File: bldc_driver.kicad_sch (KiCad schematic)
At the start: 9 parts, among them IC1 TMC6200-TA, Q1 TPH1R306PL, Q2 TPH1R306PL, Q3 TPH1R306PL, Q4 TPH1R306PL

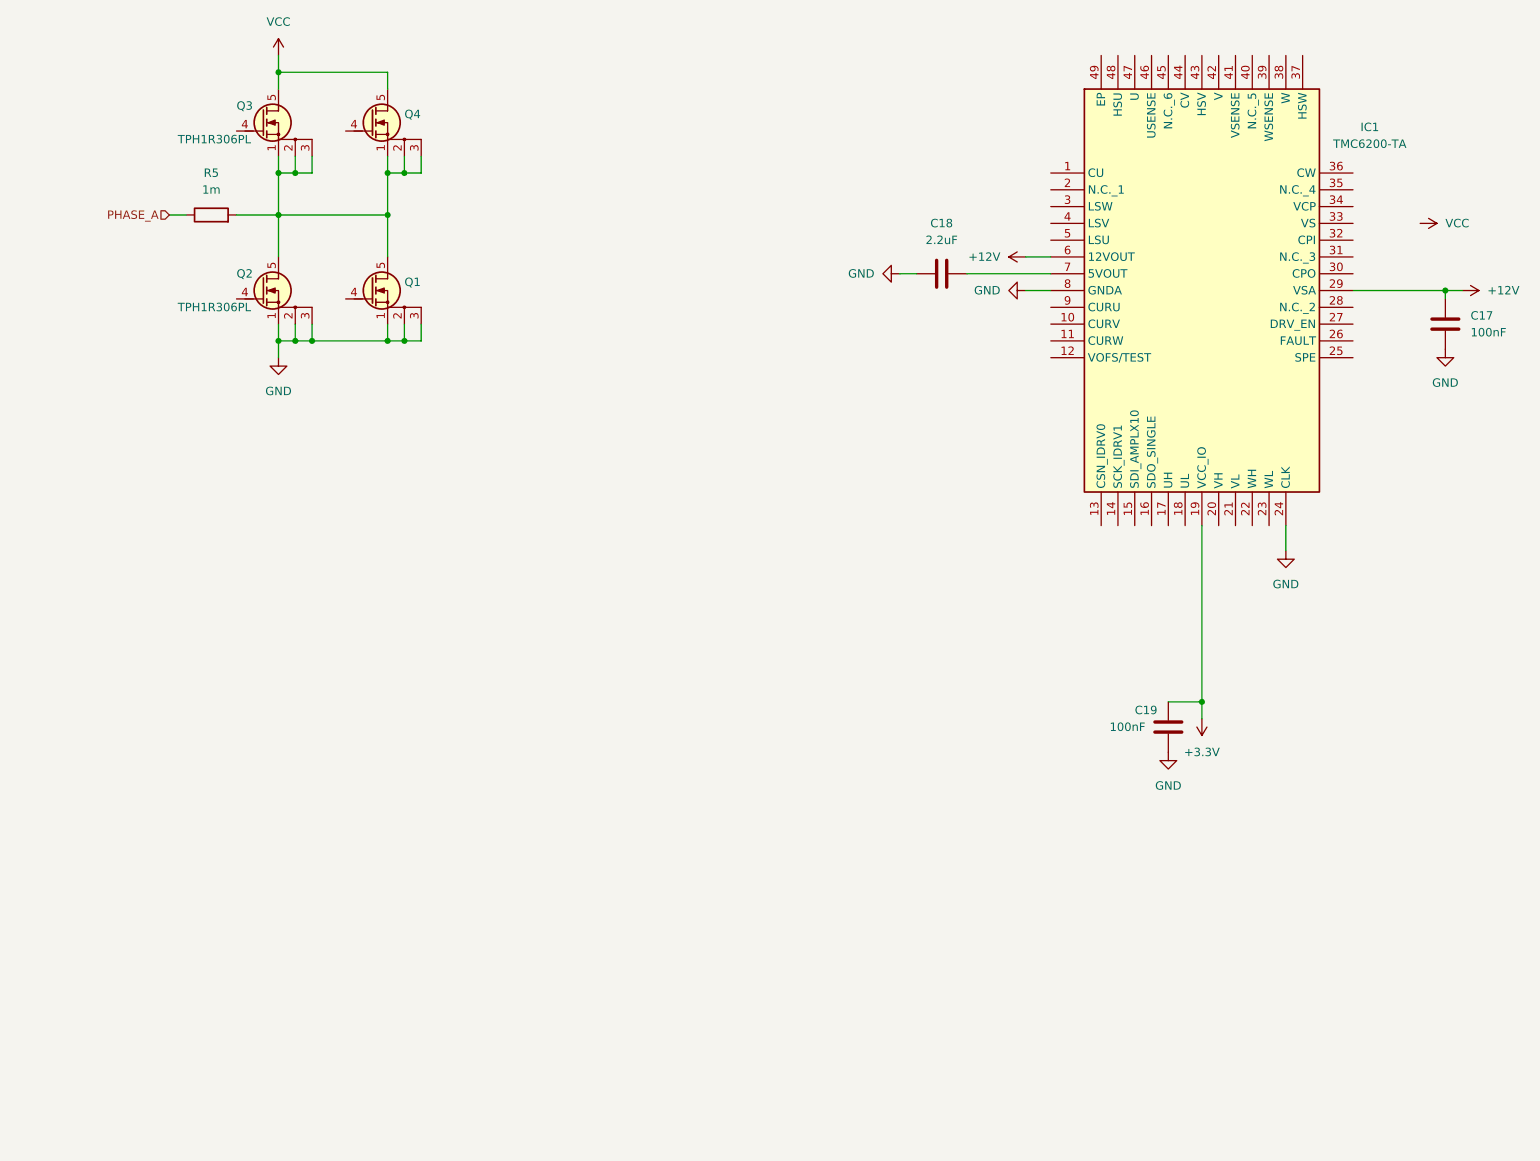
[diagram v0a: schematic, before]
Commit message: 📂 Commit before drastic power board changes
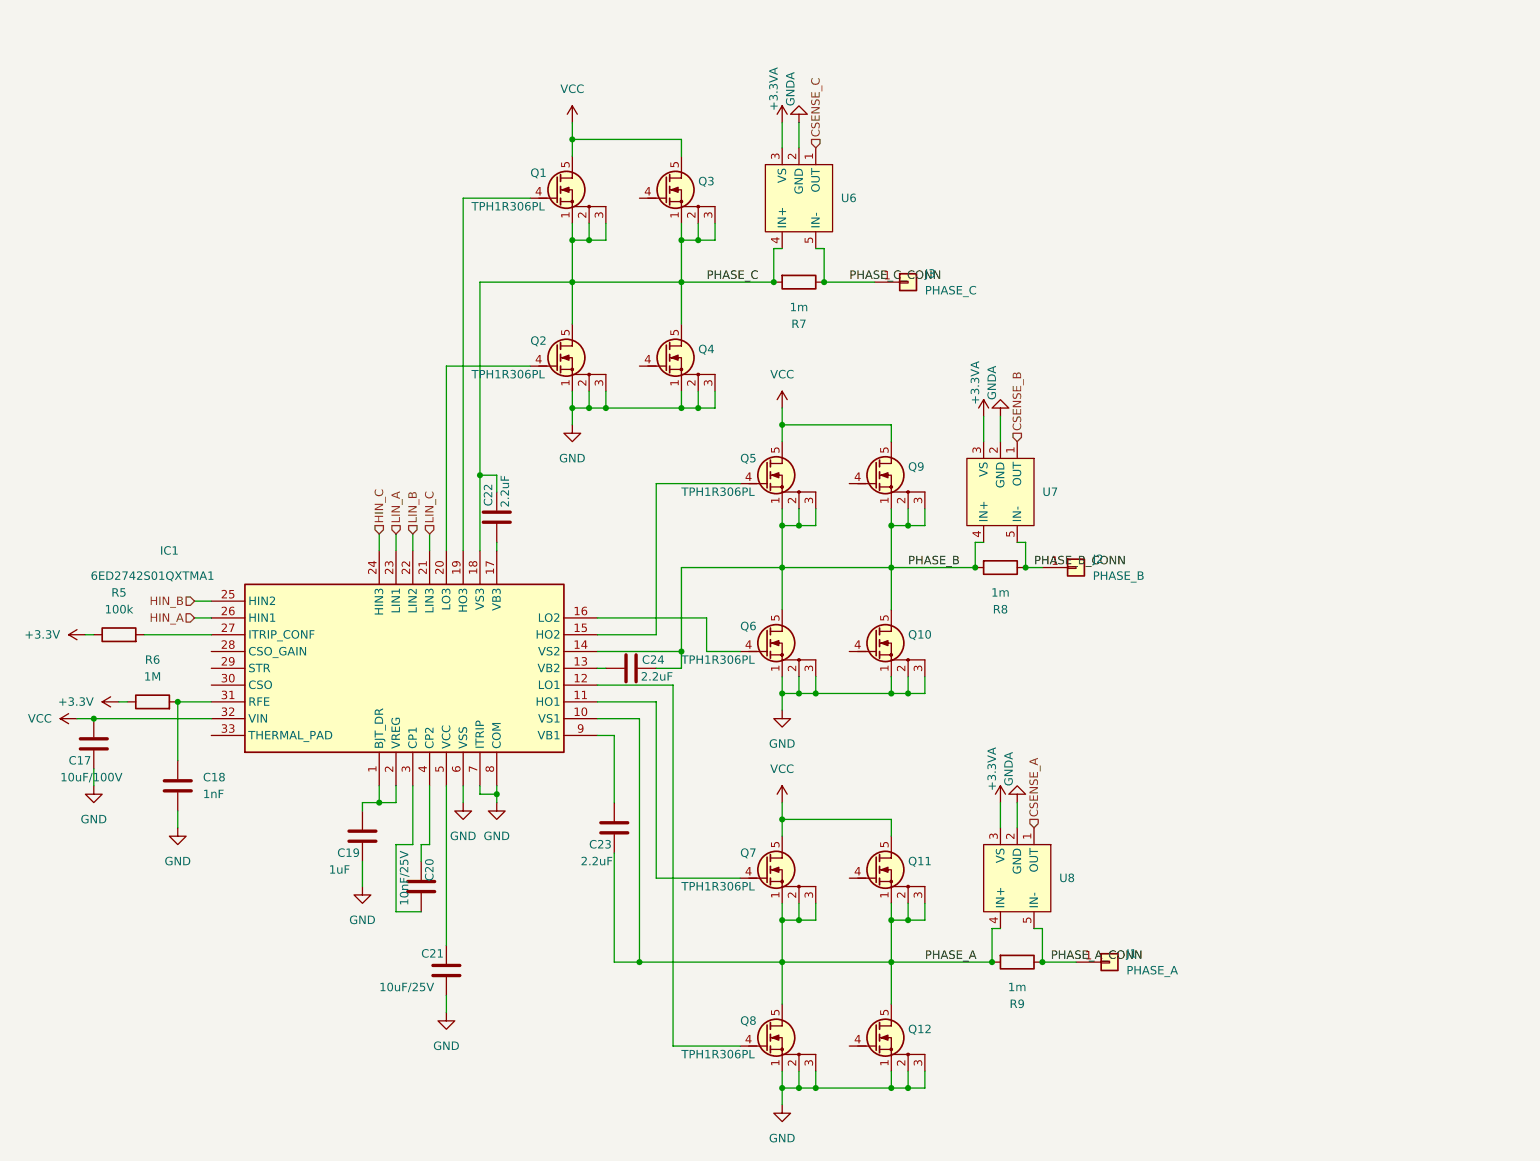
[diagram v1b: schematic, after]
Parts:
- removed IC1: TMC6200-TA, QFP50P900X900X120-49N, symbol TMC6200-TA:TMC6200-TA
- added C20: 10nF/25V, PCM_Capacitor_SMD_AKL:C_0603_1608Metric, symbol Device:C
- added C21: 10uF/25V, PCM_Capacitor_SMD_AKL:C_1206_3216Metric, symbol Device:C
- added C22, C23, C24: 2.2uF, PCM_Capacitor_SMD_AKL:C_1206_3216Metric, symbol Device:C
- added IC1: 6ED2742S01QXTMA1, CycleIQ:QFN50P500X500X90-33N-D, symbol 6ED2742S01QXTMA1:6ED2742S01QXTMA1
- added J1: PHASE_A, Connector_Wire:SolderWire-2.5sqmm_1x01_D2.4mm_OD3.6mm, symbol Connector_Generic:Conn_01x01
- added J2: PHASE_B, Connector_Wire:SolderWire-2.5sqmm_1x01_D2.4mm_OD3.6mm, symbol Connector_Generic:Conn_01x01
- added J3: PHASE_C, Connector_Wire:SolderWire-2.5sqmm_1x01_D2.4mm_OD3.6mm, symbol Connector_Generic:Conn_01x01
- added Q10, Q11, Q12, Q5, Q6, Q7, Q8, Q9: TPH1R306PL, PCM_Package_SON_AKL:Infineon_PG-TDSON-8, symbol PCM_Transistor_MOSFET_AKL:TPH1R306PL
- added R5: 100k, symbol Device:R
- added R6: 1M, symbol Device:R
- added R8, R9: 1m, PCM_Resistor_SMD_AKL:R_2512_6332Metric, symbol Device:R
- added U6, U7, U8: ~, PCM_Package_TO_SOT_SMD_AKL:SOT-353_SC-70-5, symbol CycleIQ:INA290
- C17: value 100nF -> 10uF/100V; footprint (none) -> PCM_Capacitor_SMD_AKL:C_1210_3225Metric
- C18: value 2.2uF -> 1nF; footprint (none) -> PCM_Capacitor_SMD_AKL:C_0603_1608Metric
- C19: value 100nF -> 1uF; footprint (none) -> PCM_Capacitor_SMD_AKL:C_0603_1608Metric
- R7: renamed from R5; footprint (none) -> PCM_Resistor_SMD_AKL:R_2512_6332Metric
- renumbered Q3 to Q1, Q4 to Q3, Q1 to Q4
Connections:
- net +12V is gone; now on net VCC: C17.1
- net +3.3V: now also R5.1, R6.1; no longer C19.2
- net GND: now also C19.2, C21.2, IC1.6 (VSS), IC1.7 (ITRIP), IC1.8 (COM), Q10.1 (S), Q10.2 (S), Q10.3 (S), Q12.1 (S), Q12.2 (S), Q12.3 (S), Q6.1 (S), Q6.2 (S), Q6.3 (S), Q8.1 (S), Q8.2 (S), Q8.3 (S); no longer C19.1
- net PHASE_A: now also C23.2, IC1.10 (VS1), Q11.1 (S), Q11.2 (S), Q11.3 (S), Q12.5 (D), Q7.1 (S), Q7.2 (S), Q7.3 (S), Q8.5 (D), R9.2, U8.4 (IN+); no longer R7.1
- net VCC: now also IC1.32 (VIN), Q11.5 (D), Q5.5 (D), Q7.5 (D), Q9.5 (D)
- net PHASE_C: now reaches Q1.1 (S), Q1.2 (S), Q1.3 (S), Q2.5 (D), Q3.1 (S), Q3.2 (S), Q3.3 (S), Q4.5 (D), R7.2
- net PHASE_C: now also C22.2, IC1.18 (VS3), U6.4 (IN+)
- net at C18.1: now also IC1.31 (RFE), R6.2
- net at Q1.4 (G): now also IC1.19 (HO3)
- net at Q2.4 (G): now also IC1.20 (LO3)
- new net: C20.1, IC1.3 (CP1)
- new net: C20.2, IC1.4 (CP2)
- new net: IC1.15 (HO2), Q5.4 (G)
- new net: IC1.11 (HO1), Q7.4 (G)
- new net: C21.1, IC1.5 (VCC)
- new net: C24.1, IC1.13 (VB2)
- new net: C23.1, IC1.9 (VB1)
- new net: IC1.16 (LO2), Q6.4 (G)
- new net: C19.1, IC1.1 (BJT_DR), IC1.2 (VREG)
- new net: C22.1, IC1.17 (VB3)
- new net: IC1.12 (LO1), Q8.4 (G)
- new net: IC1.27 (ITRIP_CONF), R5.2
- new net +3.3VA: U6.3 (VS), U7.3 (VS), U8.3 (VS)
- new net CSENSE_A: U8.1 (OUT)
- new net CSENSE_B: U7.1 (OUT)
- new net CSENSE_C: U6.1 (OUT)
- new net GNDA: U6.2 (GND), U7.2 (GND), U8.2 (GND)
- new net HIN_A: IC1.26 (HIN1)
- new net HIN_B: IC1.25 (HIN2)
- new net HIN_C: IC1.24 (HIN3)
- new net LIN_A: IC1.23 (LIN1)
- new net LIN_B: IC1.22 (LIN2)
- new net LIN_C: IC1.21 (LIN3)
- new net PHASE_A_CONN: J1.1 (Pin_1), R9.1, U8.5 (IN-)
- new net PHASE_B: C24.2, IC1.14 (VS2), Q10.5 (D), Q5.1 (S), Q5.2 (S), Q5.3 (S), Q6.5 (D), Q9.1 (S), Q9.2 (S), Q9.3 (S), R8.2, U7.4 (IN+)
- new net PHASE_B_CONN: J2.1 (Pin_1), R8.1, U7.5 (IN-)
- new net PHASE_C_CONN: J3.1 (Pin_1), R7.1, U6.5 (IN-)
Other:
- moved on the sheet: Q1, Q2, Q3, Q4, R7
